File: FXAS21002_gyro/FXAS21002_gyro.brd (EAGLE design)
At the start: 15.2 x 15.2 mm, 9 parts

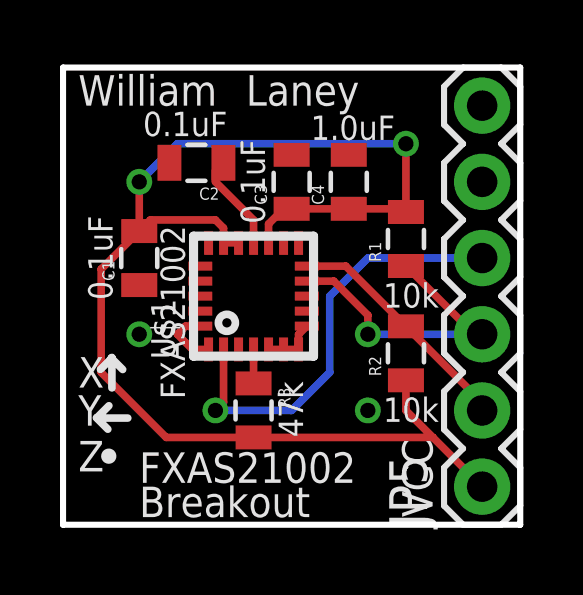
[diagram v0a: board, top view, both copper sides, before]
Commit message: prep for fab
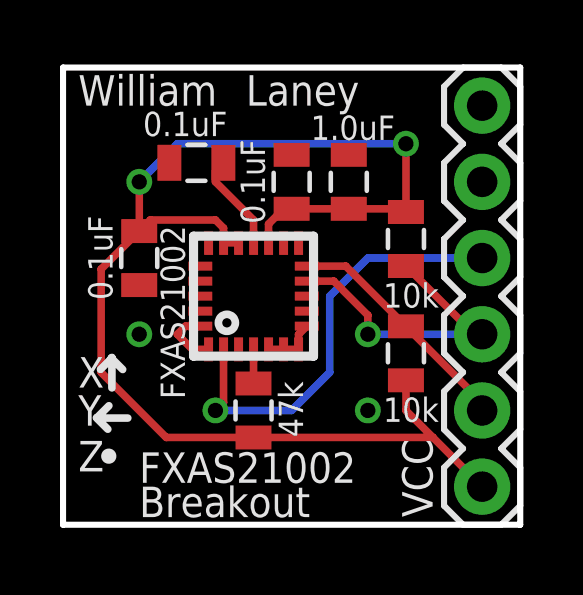
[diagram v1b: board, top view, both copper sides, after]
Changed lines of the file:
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@@
 <setting verticaltext="up"/>
 </settings>
-<grid distance="0.005" unitdist="inch" unit="inch" style="lines" multiple="1" display="yes" altdistance="0.005" altunitdist="inch" altunit="inch"/>
+<grid distance="0.05" unitdist="inch" unit="inch" style="lines" multiple="1" display="yes" altdistance="0.005" altunitdist="inch" altunit="inch"/>
 <layers>
 <layer number="1" name="Top" color="4" fill="1" visible="yes" active="yes"/>
@@
 <layer number="23" name="tOrigins" color="15" fill="1" visible="yes" active="yes"/>
 <layer number="24" name="bOrigins" color="15" fill="1" visible="yes" active="yes"/>
-<layer number="25" name="tNames" color="7" fill="1" visible="no" active="yes"/>
+<layer number="25" name="tNames" color="7" fill="1" visible="yes" active="yes"/>
 <layer number="26" name="bNames" color="7" fill="1" visible="no" active="yes"/>
-<layer number="27" name="tValues" color="7" fill="1" visible="no" active="yes"/>
+<layer number="27" name="tValues" color="7" fill="1" visible="yes" active="yes"/>
 <layer number="28" name="bValues" color="7" fill="1" visible="no" active="yes"/>
 <layer number="29" name="tStop" color="7" fill="3" visible="no" active="yes"/>
@@
 </autorouter>
 <elements>
-<element name="C1" library="SparkFun-Passives" package="0805" value="0.1uF" x="2.54" y="8.89" rot="R90"/>
-<element name="C2" library="SparkFun-Passives" package="0805" value="0.1uF" x="4.445" y="12.065" rot="R180"/>
-<element name="C3" library="SparkFun-Passives" package="0805" value="0.1uF" x="7.62" y="11.43" rot="R90"/>
-<element name="C4" library="SparkFun-Passives" package="0805" value="1.0uF" x="9.525" y="11.43" rot="R90"/>
-<element name="JP5" library="SparkFun" package="1X06" value="" x="13.97" y="1.27" rot="R90"/>
-<element name="R1" library="SparkFun-Passives" package="0805" value="10k" x="11.43" y="9.525" rot="R90"/>
-<element name="R2" library="SparkFun-Passives" package="0805" value="10k" x="11.43" y="5.715" rot="R90"/>
-<element name="R3" library="SparkFun-Passives" package="0805" value="47k" x="6.35" y="3.81" rot="R270"/>
-<element name="U$1" library="sharkdunio" package="24QFN" value="FXAS21002" x="6.35" y="7.62" rot="R90"/>
+<element name="C1" library="SparkFun-Passives" package="0805" value="0.1uF" x="2.54" y="8.89" smashed="yes" rot="R90"/>
+<element name="C2" library="SparkFun-Passives" package="0805" value="0.1uF" x="4.445" y="12.065" smashed="yes" rot="R180"/>
+<element name="C3" library="SparkFun-Passives" package="0805" value="0.1uF" x="7.62" y="11.43" smashed="yes" rot="R90"/>
+<element name="C4" library="SparkFun-Passives" package="0805" value="1.0uF" x="9.525" y="11.43" smashed="yes" rot="R90"/>
+<element name="JP5" library="SparkFun" package="1X06" value="" x="13.97" y="1.27" smashed="yes" rot="R90">
+<attribute name="VALUE" x="17.145" y="0" size="1.27" layer="27" rot="R90"/>
+</element>
+<element name="R1" library="SparkFun-Passives" package="0805" value="10k" x="11.43" y="9.525" smashed="yes" rot="R90"/>
+<element name="R2" library="SparkFun-Passives" package="0805" value="10k" x="11.43" y="5.715" smashed="yes" rot="R90"/>
+<element name="R3" library="SparkFun-Passives" package="0805" value="47k" x="6.35" y="3.81" smashed="yes" rot="R270"/>
+<element name="U$1" library="sharkdunio" package="24QFN" value="FXAS21002" x="6.35" y="7.62" smashed="yes" rot="R90"/>
 </elements>
 <signals>
